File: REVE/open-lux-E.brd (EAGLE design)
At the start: 55.4 x 62 mm, 54 parts, among them IC1 24AA128SN, IC2 MCP73831, IC3 ATMEGA32U4-AU, IC4 MCP1700-33, J1 AYZ0202, Q4 BSS123, T1 FDN340P, T2 FDN340P, X2 USBSMD, X3 8MHz

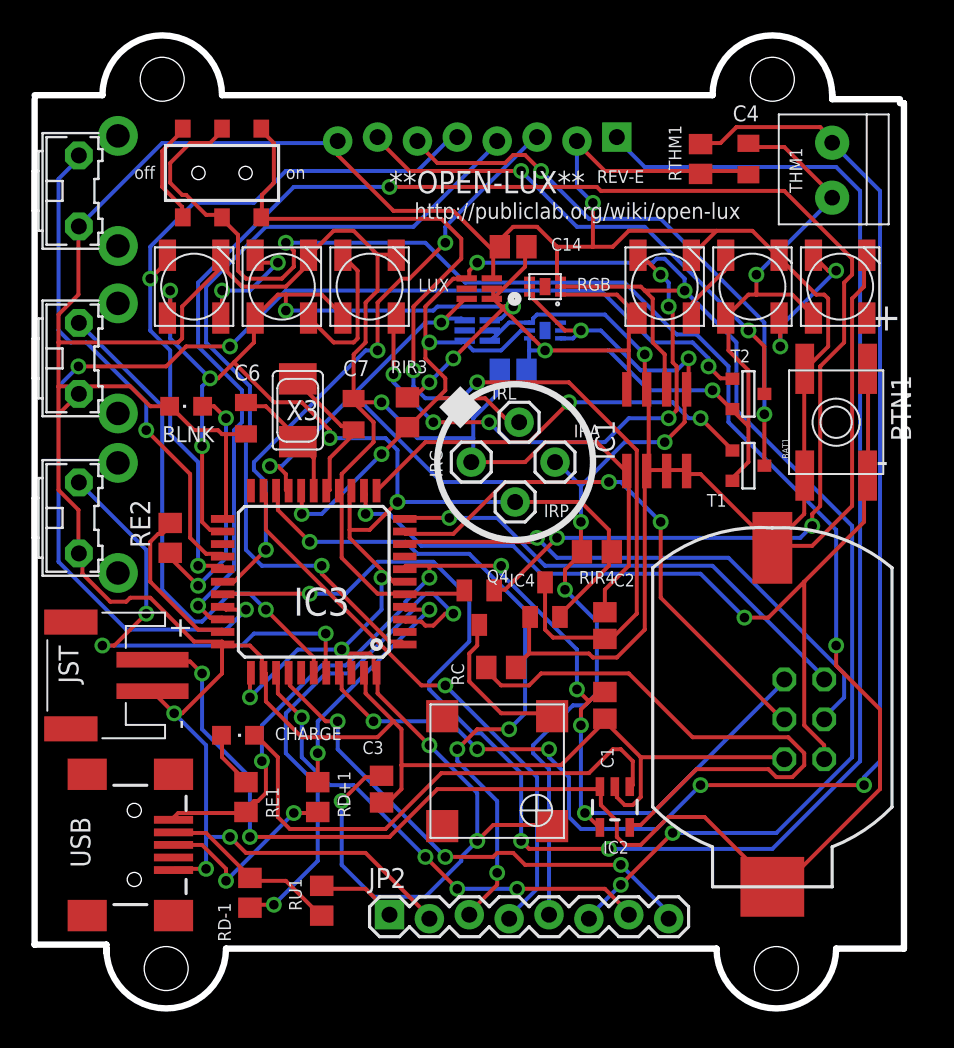
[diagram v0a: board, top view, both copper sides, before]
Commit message: update
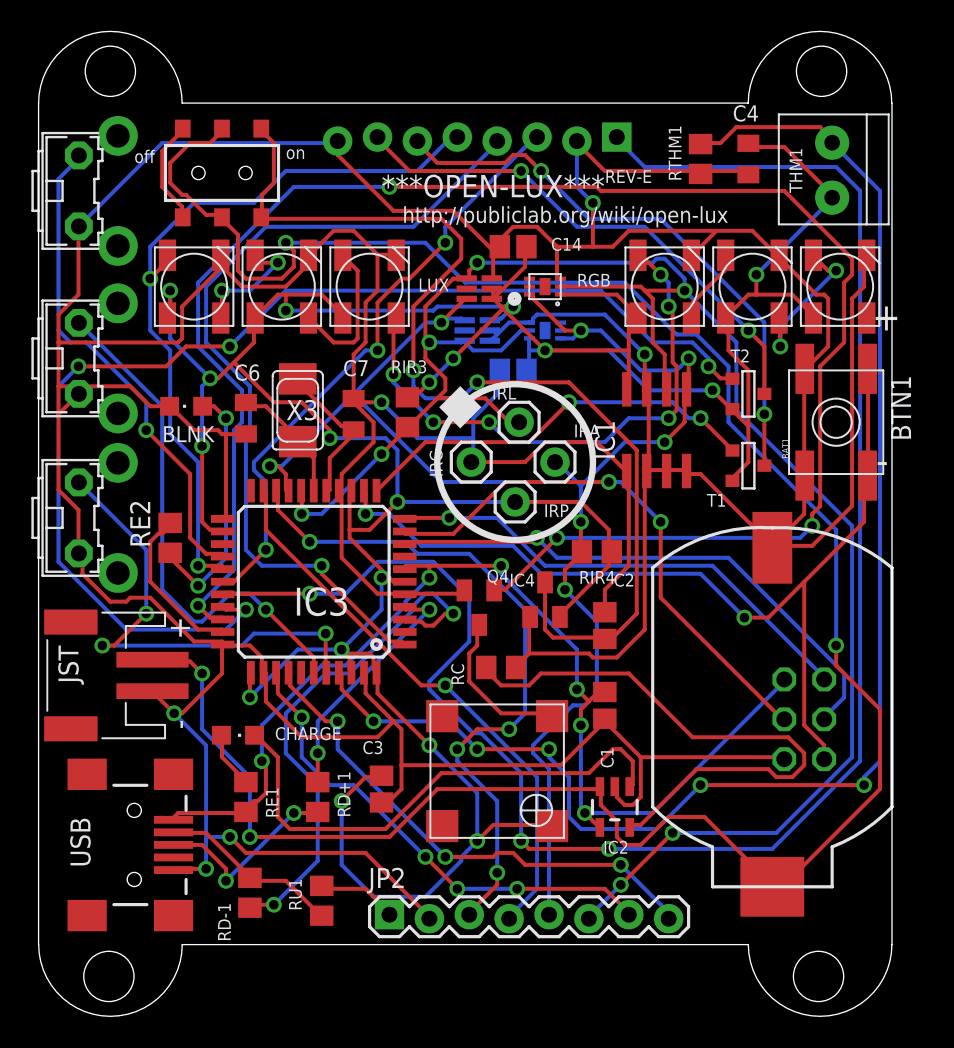
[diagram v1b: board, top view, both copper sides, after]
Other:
- board size 55.4 x 62 mm -> 54.4 x 62.7 mm
- board text added: "***OPEN-LUX***"
- board text removed: "**OPEN-LUX**"
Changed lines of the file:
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@@
 <setting verticaltext="up"/>
 </settings>
-<grid distance="0.01" unitdist="inch" unit="inch" style="lines" multiple="1" display="no" altdistance="0.025" altunitdist="inch" altunit="inch"/>
+<grid distance="0.05" unitdist="mm" unit="mm" style="lines" multiple="1" display="no" altdistance="0.025" altunitdist="inch" altunit="inch"/>
 <layers>
 <layer number="1" name="Top" color="4" fill="1" visible="yes" active="yes"/>
@@
 <text x="53.34" y="29.972" size="1.778" layer="21">-</text>
 <text x="51.816" y="17.272" size="0.8128" layer="22" rot="MR180">GND</text>
-<text x="17.272" y="52.07" size="0.8128" layer="22" rot="MR0">NOKIA 5110</text>
+<text x="17.272" y="51.562" size="0.8128" layer="22" rot="MR0">NOKIA 5110</text>
 <text x="40.132" y="43.942" size="0.8128" layer="22" rot="MR270">A1</text>
 <text x="51.562" y="14.732" size="0.8128" layer="22" rot="MR180">MOSI</text>
@@
 <text x="41.91" y="17.272" size="0.8128" layer="22" rot="MR180">RESET</text>
 <text x="54.102" y="51.816" size="1.4224" layer="22" font="vector" rot="MR270">publiclab.org/wiki/open-lux</text>
-<wire x1="54.864" y1="53.594" x2="55.118" y2="53.594" width="0.4064" layer="20"/>
-<wire x1="55.118" y1="53.594" x2="55.118" y2="-0.254" width="0.4064" layer="20"/>
-<wire x1="4.318" y1="-0.254" x2="4.318" y2="-0.508" width="0.4064" layer="20"/>
-<wire x1="11.938" y1="-0.254" x2="4.318" y2="-0.254" width="0.4064" layer="20" curve="-180"/>
-<wire x1="50.8" y1="-0.254" x2="43.18" y2="-0.254" width="0.4064" layer="20" curve="-180"/>
-<hole x="8.128" y="-1.524" drill="2.8"/>
-<hole x="46.99" y="-1.524" drill="2.8"/>
-<wire x1="-0.254" y1="0" x2="4.318" y2="0" width="0.4064" layer="20"/>
-<wire x1="4.318" y1="0" x2="4.318" y2="-0.254" width="0.4064" layer="20"/>
-<wire x1="11.938" y1="-0.254" x2="43.18" y2="-0.254" width="0.4064" layer="20"/>
-<wire x1="50.8" y1="-0.254" x2="55.118" y2="-0.254" width="0.4064" layer="20"/>
-<wire x1="-0.254" y1="0" x2="-0.254" y2="53.848" width="0.4064" layer="20"/>
-<wire x1="50.546" y1="54.102" x2="50.546" y2="54.356" width="0.4064" layer="20"/>
-<wire x1="42.926" y1="54.102" x2="50.546" y2="54.102" width="0.4064" layer="20" curve="-180"/>
-<wire x1="4.064" y1="54.102" x2="11.684" y2="54.102" width="0.4064" layer="20" curve="-180"/>
-<hole x="46.736" y="55.118" drill="2.8"/>
-<hole x="7.874" y="55.118" drill="2.8"/>
-<wire x1="54.864" y1="53.848" x2="50.546" y2="53.848" width="0.4064" layer="20"/>
-<wire x1="50.546" y1="53.848" x2="50.546" y2="54.102" width="0.4064" layer="20"/>
-<wire x1="42.926" y1="54.102" x2="11.684" y2="54.102" width="0.4064" layer="20"/>
-<wire x1="4.064" y1="54.102" x2="-0.254" y2="54.102" width="0.4064" layer="20"/>
-<text x="34.798" y="49.276" size="1.4224" layer="21" font="vector" rot="R180">**OPEN-LUX**</text>
+<text x="36.068" y="49.022" size="1.4224" layer="21" font="vector" rot="R180">***OPEN-LUX***</text>
 <text x="2.032" y="8.128" size="1.27" layer="21" font="vector" rot="R270">USB</text>
 <text x="1.27" y="19.05" size="1.27" layer="21" font="vector" rot="R270">JST</text>
 <text x="26.162" y="42.418" size="0.8128" layer="21" font="vector" rot="R180">LUX</text>
-<text x="34.29" y="41.656" size="0.8128" layer="21" font="vector">RGB</text>
+<text x="34.29" y="41.91" size="0.8128" layer="21" font="vector">RGB</text>
 <text x="25.908" y="38.862" size="0.8128" layer="22" rot="MR0">LUX</text>
-<text x="36.322" y="38.608" size="0.8128" layer="22" rot="MR0">RGB</text>
-<text x="44.704" y="47.244" size="1.016" layer="21" font="vector" rot="R180">http://publiclab.org/wiki/open-lux</text>
-<text x="35.56" y="48.514" size="0.8128" layer="21" font="vector">REV-E</text>
-<text x="15.748" y="48.768" size="0.8128" layer="21" font="vector">on</text>
-<text x="6.096" y="48.768" size="0.8128" layer="21" font="vector">off</text>
+<text x="36.322" y="38.862" size="0.8128" layer="22" rot="MR0">RGB</text>
+<text x="43.942" y="46.99" size="1.016" layer="21" font="vector" rot="R180">http://publiclab.org/wiki/open-lux</text>
+<text x="36.068" y="48.514" size="0.8128" layer="21" font="vector">REV-E</text>
+<text x="15.748" y="50.038" size="0.8128" layer="21" font="vector">on</text>
+<text x="6.096" y="49.784" size="0.8128" layer="21" font="vector">off</text>
+<hole x="4.572" y="55.626" drill="3.2"/>
+<wire x1="54.356" y1="53.594" x2="54.356" y2="0" width="0" layer="20"/>
+<wire x1="0" y1="0" x2="0" y2="53.594" width="0" layer="20"/>
+<wire x1="0" y1="53.594" x2="9.144" y2="53.594" width="0" layer="20" curve="-180"/>
+<hole x="49.872" y="55.626" drill="3.2"/>
+<wire x1="45.2" y1="53.594" x2="54.344" y2="53.594" width="0" layer="20" curve="-180"/>
+<hole x="4.478" y="-2.026" drill="3.2"/>
+<wire x1="9.15" y1="0.006" x2="0.006" y2="0.006" width="0" layer="20" curve="-180"/>
+<hole x="49.678" y="-2.026" drill="3.2"/>
+<wire x1="54.35" y1="0.006" x2="45.206" y2="0.006" width="0" layer="20" curve="-180"/>
+<wire x1="45.2" y1="0" x2="9.15" y2="0" width="0" layer="20"/>
+<wire x1="45.2" y1="53.6" x2="9.15" y2="53.6" width="0" layer="20"/>
 </plain>
 <attributes>
